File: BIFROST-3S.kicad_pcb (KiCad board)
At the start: 2 copper layers, 60 x 40 mm, 6 parts, among them J1 1-776267-1, J2 200241-1222, J3 200241-1222, J4 B6B-XH-A_LF__SN_, J5 B4B-XH-A_LF__SN_

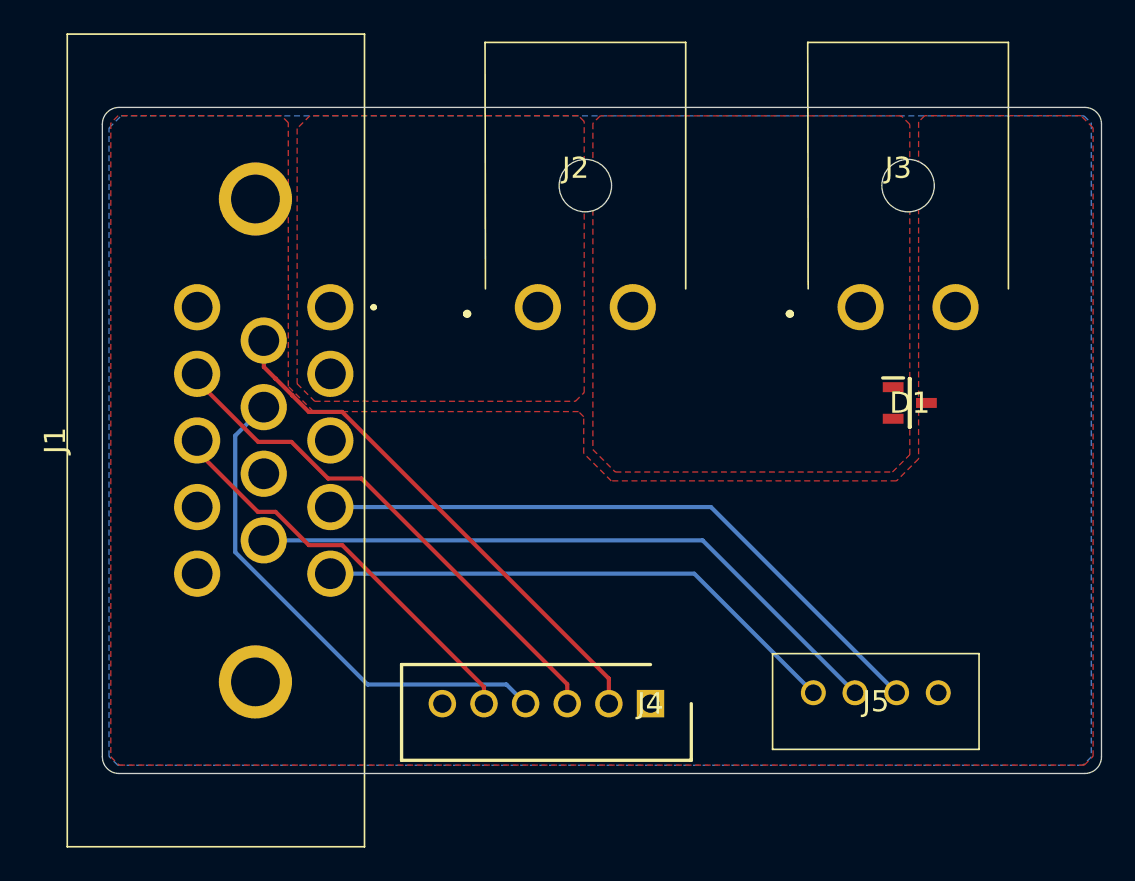
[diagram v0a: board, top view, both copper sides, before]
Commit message: Schematic+Layout 2.0
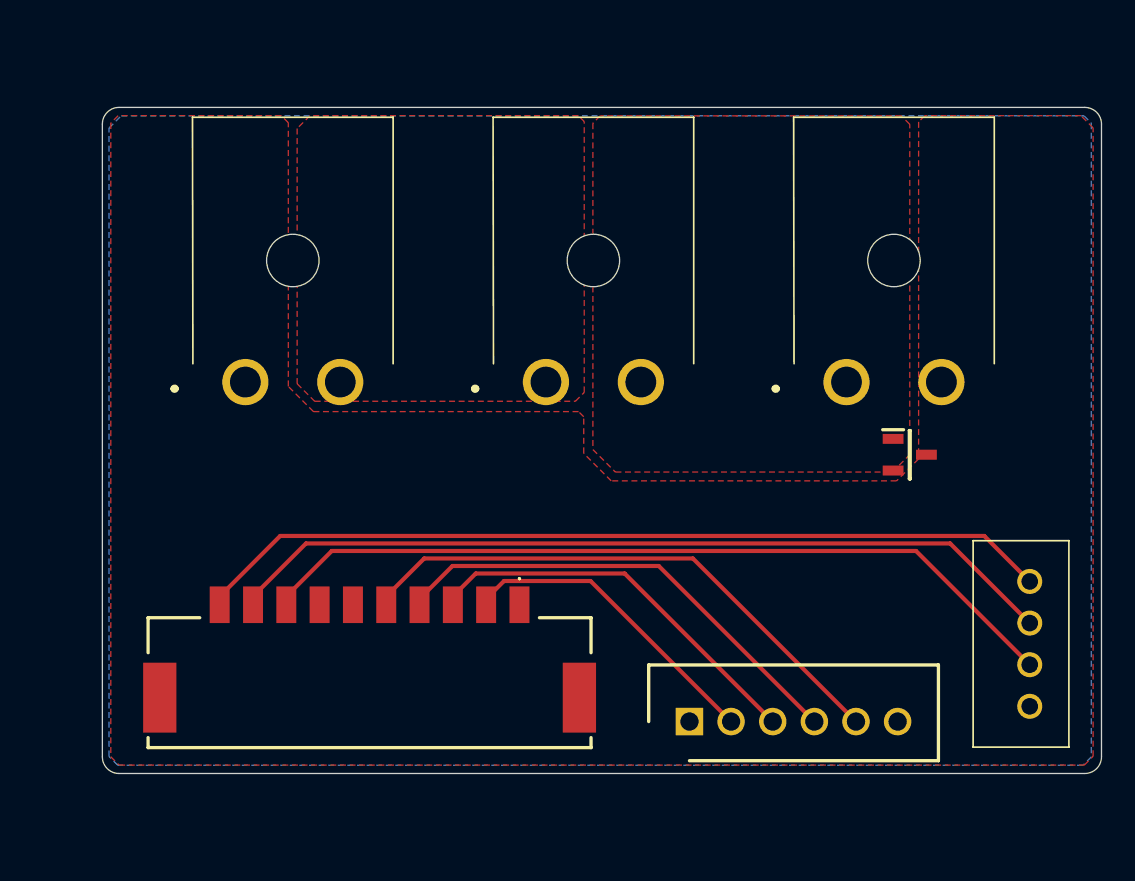
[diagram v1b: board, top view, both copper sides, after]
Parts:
- removed J1: 1-776267-1, 1-776267-1:17762671
- added J6: 560020-1020, 560020-1020:5600201020, F.Cu at (131.4, 112.3)
- added J7: 200241-1222, 200241-1222:2002411222, F.Cu at (123.9, 94.3)
- moved J5 5.56 mm to (171.0, 113.7), turned to 90 degrees
- moved J3 4.58 mm to (160.0, 94.3)
- moved J2 4.52 mm to (142.0, 94.3)
- moved D1 3.11 mm to (163.8, 98.6)
- moved J4 2.58 mm to (150.6, 114.6), turned to 0 degrees
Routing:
- net /BQ2_TS1: track 32.0 -> 51.8 mm
- net /BAT1: track 31.6 -> 19.0 mm
- net /BQ2_TS2: track 39.3 -> 50.4 mm
- net /BQ2_TS3: track 38.6 -> 49.1 mm
- net /BQ_TS: track 24.7 -> 33.7 mm
- net /BAT2: track 31.4 -> 24.0 mm
- net /BAT3: track 30.6 -> 28.8 mm
